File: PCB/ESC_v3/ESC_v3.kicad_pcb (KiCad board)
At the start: 4 copper layers, 42 x 83.5 mm, 144 parts, among them J1 Conn_01x04_Pin, J10 Conn_01x01_Pin, J11 Screw_Terminal_01x01, J2 Screw_Terminal_01x01, J3 Conn_01x01_Pin, J4 Conn_01x01_Pin, J5 Conn_01x01_Pin, J6 Conn_01x01_Pin, J7 Conn_01x01_Pin, J8 Conn_01x01_Pin, J9 Conn_01x01_Pin, Q1 NTMFS2D1N08XT1G, Q2 NTMFS2D1N08XT1G, Q3 NTMFS2D1N08XT1G, Q4 NTMFS2D1N08XT1G, Q5 NTMFS2D1N08XT1G, Q6 NTMFS2D1N08XT1G, U1 SN65HVD232, U2 DRV8323SRTAT, U3 STM32G474CETx, Y2 24MHz

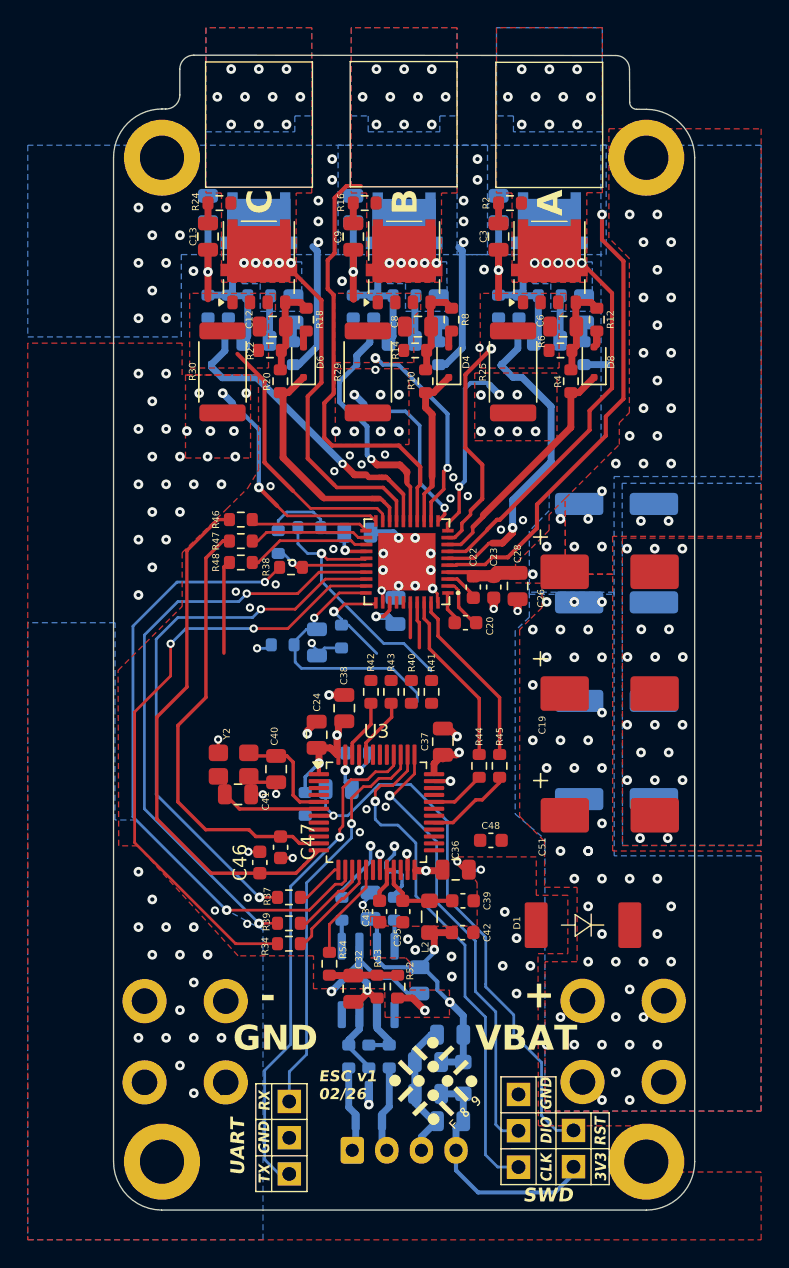
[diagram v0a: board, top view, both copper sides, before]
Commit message: Layout edit
Changed some layout and optimized
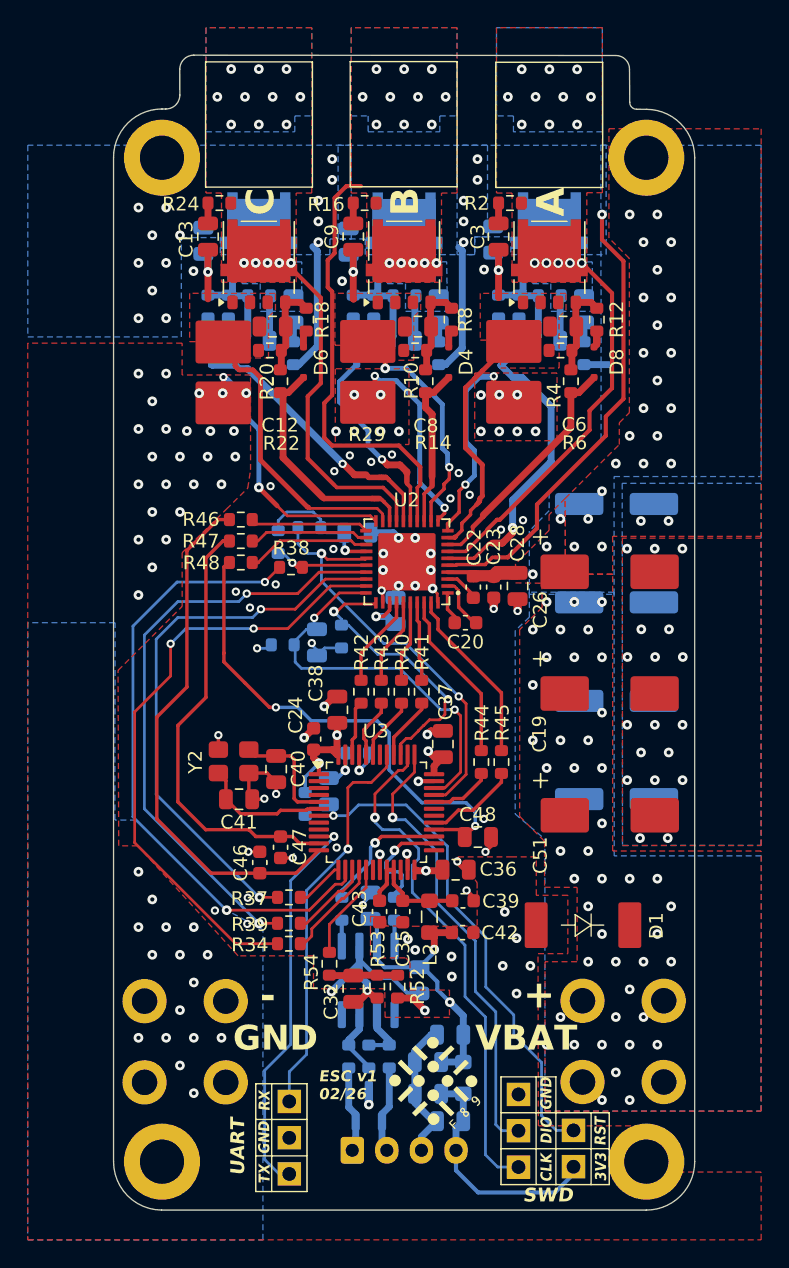
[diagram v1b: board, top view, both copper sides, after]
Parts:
- C24: footprint Capacitor_SMD:C_0805_2012Metric -> Capacitor_SMD:C_0603_1608Metric
- C48: footprint Capacitor_SMD:C_0603_1608Metric -> Capacitor_SMD:C_0805_2012Metric
- moved NT2 2.57 mm to (144.2, 53.5), turned to 180 degrees
- moved C15 2.38 mm to (141.2, 43.5)
- moved C18 2.32 mm to (130.7, 43.4)
- moved C4 2.24 mm to (151.6, 43.3)
- moved NT3 1.20 mm to (132.6, 53.6)
- moved NT1 1.09 mm to (151.2, 53.2), turned to 0 degrees
- moved C48 0.97 mm to (150.5, 86.5)
- moved C33 0.73 mm to (139.8, 83.2), turned to 90 degrees
- moved R40 0.71 mm to (145.0, 76.0)
- moved R41 0.71 mm to (146.5, 76.0)
- moved R42 0.71 mm to (142.1, 76.0)
- moved R43 0.71 mm to (143.6, 76.0)
- moved C38 0.52 mm to (140.4, 77.3)
- moved C24 0.38 mm to (138.7, 79.4)
- moved C41 0.36 mm to (133.3, 83.8)
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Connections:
- U3 pad 33: unconnected-(U3-PA11-Pad33) -> NFAULT
- U3 pad 34: unconnected-(U3-PA12-Pad34) -> ENABLE
- U3 pad 39: unconnected-(U3-PA15-Pad39) -> CAL
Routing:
- net ADC4_IN4: track 6.76 -> 35.8 mm, vias 0 -> 2
- net CAL: track 7.91 -> 20.5 mm, vias 1 -> 2
- net NFAULT: track 19.2 -> 30.8 mm, vias 1 -> 2
- net ENABLE: track 19.3 -> 29.0 mm, vias 1 -> 2
- net USART2_TX: track 36.5 -> 28.7 mm
- net SPA: track 27.5 -> 20.3 mm, vias 2 -> 1
- net INHA: track 0.00 -> 6.69 mm
- net INLA: track 0.00 -> 6.29 mm
- net CAN_TX: track 4.58 -> 9.39 mm
- net TIM8_CH1: track 0.00 -> 4.58 mm
- net TIM8_CH1N: track 0.00 -> 4.56 mm
- net GND: track 62.2 -> 66.7 mm, vias 141 -> 140
- net NRST: track 42.4 -> 38.9 mm
- net INHB: track 2.55 -> 5.90 mm
- net CAN_RX: track 5.07 -> 7.83 mm
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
